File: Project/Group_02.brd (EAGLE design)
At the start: 71.1 x 41.9 mm, 29 parts, among them J1 POWER_JACKPTH_LOCK, U1 +12v

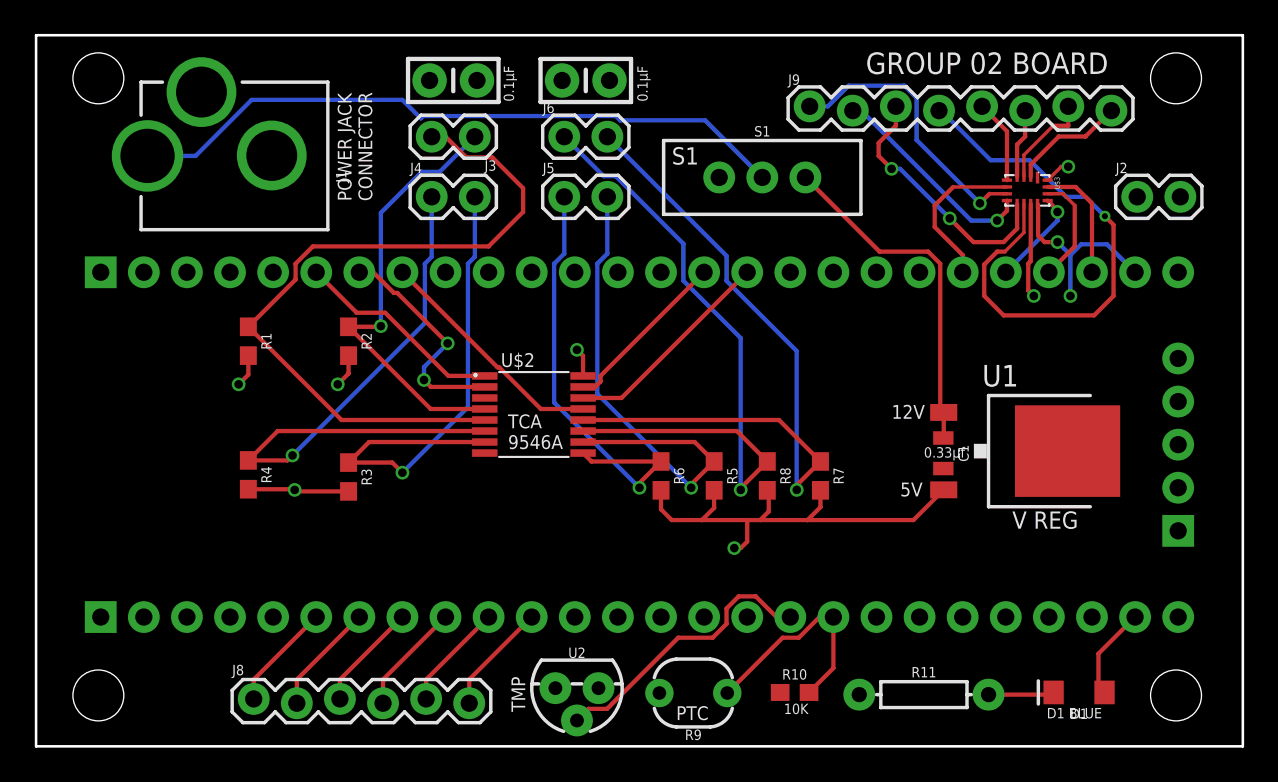
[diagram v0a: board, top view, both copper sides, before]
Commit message: File completi
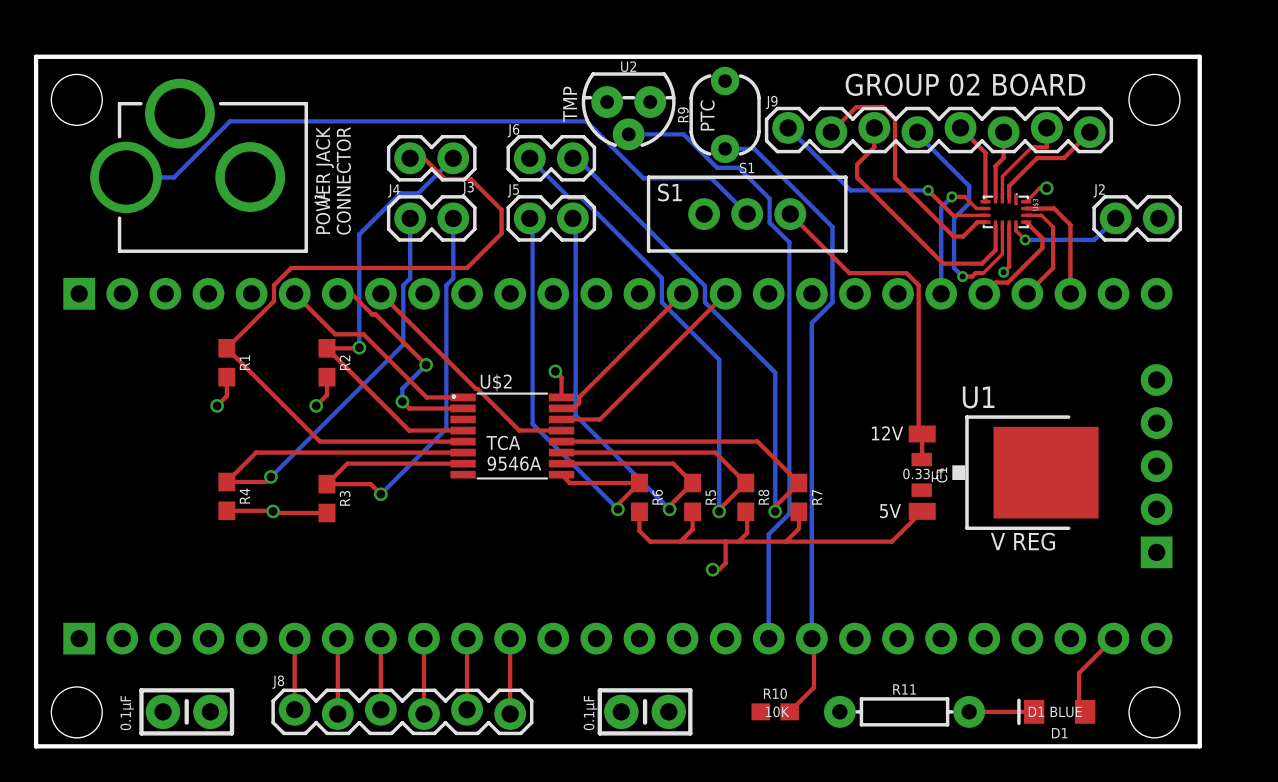
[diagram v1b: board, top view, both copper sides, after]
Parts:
- moved C3 44.0 mm to (8.88, 2.03), turned to 180 degrees
- moved C2 38.9 mm to (35.9, 2.03)
- moved U2 34.7 mm to (34.9, 38.0)
- moved R9 34.1 mm to (40.6, 37.2), turned to 90 degrees
- moved J8 2.50 mm to (15.2, 2.16)
- moved J6 2.40 mm to (29.1, 34.7)
- moved J5 2.40 mm to (29.1, 31.1)
- moved S1 2.33 mm to (41.9, 31.4)
- moved J1 1.80 mm to (19.2, 33.5)
- moved J2 1.80 mm to (63.6, 31.1)
- moved J3 1.80 mm to (24.6, 34.7)
- moved R5 1.80 mm to (38.7, 14.7)
- moved R7 1.80 mm to (45.0, 14.7)
- moved R8 1.80 mm to (41.8, 14.7)
- moved U$3 1.80 mm to (57.1, 31.5)
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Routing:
- net PHOTO_OUT: track 13.1 -> 38.0 mm
- net TEMP_OUT: track 16.6 -> 36.8 mm
- net N$14: track 32.5 -> 14.9 mm
- net GND: track 11.4 -> 6.94 mm, vias 2 -> 1
- net N$17: track 16.7 -> 13.8 mm
- net 5V: track 45.8 -> 43.1 mm
- net N$16: track 12.6 -> 15.2 mm, vias 1 -> 0
- net N$6: track 6.35 -> 4.19 mm
- net N$2: track 6.35 -> 4.19 mm
- net N$7: track 6.61 -> 4.44 mm
- net N$5: track 6.61 -> 4.44 mm
- net N$4: track 6.35 -> 4.19 mm
- net N$3: track 6.61 -> 4.44 mm
- net MUX_OUT: track 9.33 -> 8.24 mm, vias 0 -> 1
- net 12V: track 20.4 -> 19.7 mm
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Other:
- board size 71.1 x 41.9 mm -> 68.6 x 40.6 mm
